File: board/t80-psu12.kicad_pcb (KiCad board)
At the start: 2 copper layers, 26 x 80 mm, 28 parts, among them J1 Conn_01x02_Female, U1 FR8205, U2 FR8205

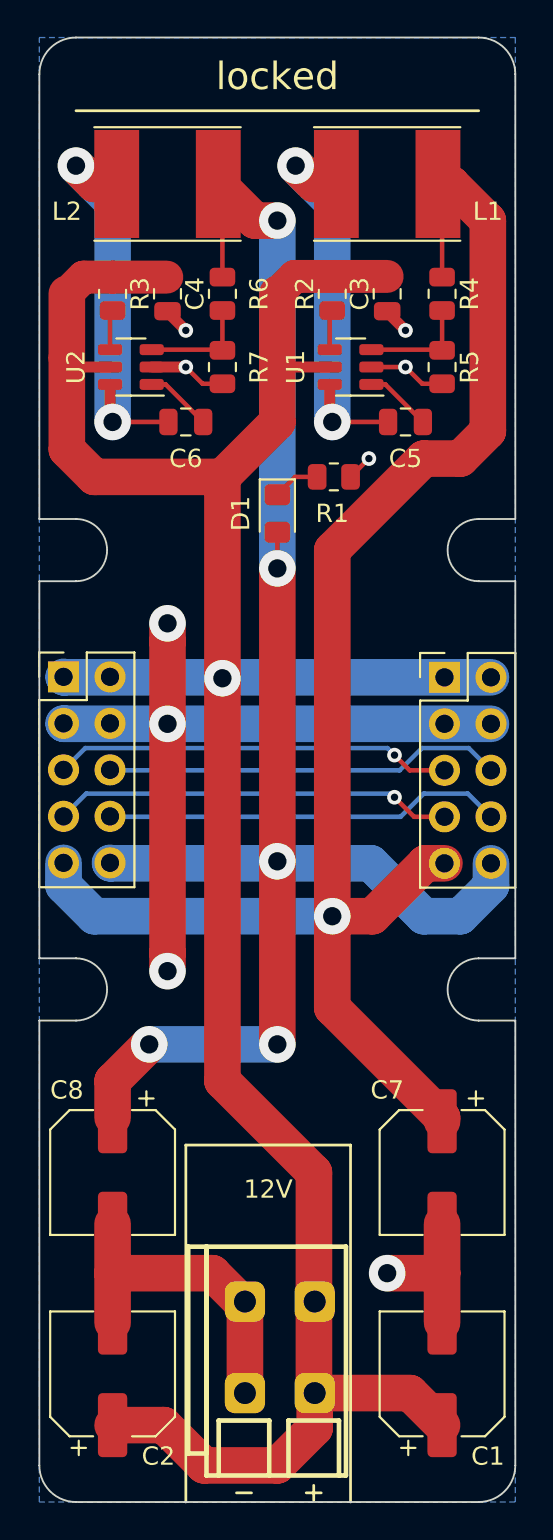
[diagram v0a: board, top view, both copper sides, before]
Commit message: WIP
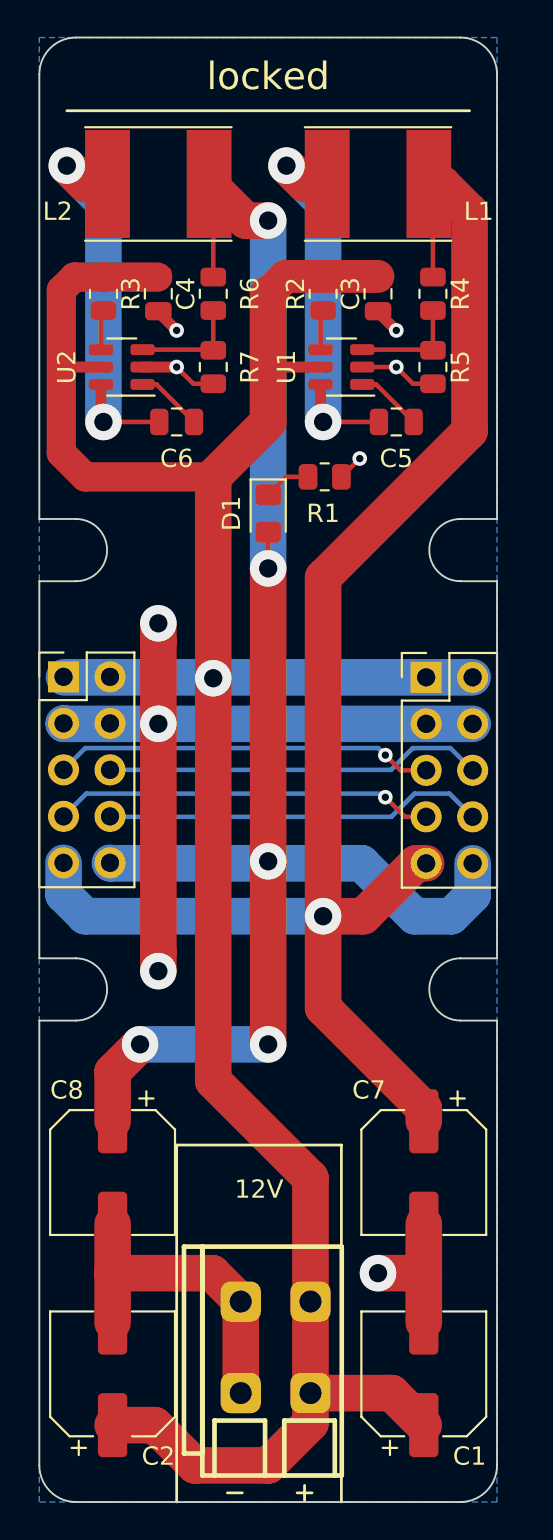
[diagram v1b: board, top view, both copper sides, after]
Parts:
- moved C1 1.00 mm to (106.0, 133.0)
- moved C7 1.00 mm to (106.0, 122.0)
- moved X2 1.00 mm to (106.1, 95.0)
- moved C3 0.50 mm to (103.5, 74.0)
- moved C4 0.50 mm to (91.5, 74.0)
- moved C5 0.50 mm to (104.5, 81.0)
- moved C6 0.50 mm to (92.5, 81.0)
- moved D1 0.50 mm to (97.5, 86.0)
- moved L1 0.50 mm to (103.5, 68.0)
- moved L2 0.50 mm to (91.5, 68.0)
- moved NT1 0.50 mm to (94.5, 95.0)
- moved NT2 0.50 mm to (100.5, 108.0)
- moved NT3 0.50 mm to (97.5, 105.0)
- moved NT4 0.50 mm to (91.5, 97.5)
- moved NT5 0.50 mm to (91.5, 97.5)
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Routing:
- net +5V: track 65.1 -> 63.3 mm
- net +12V: track 121.0 -> 119.3 mm
- net /PWR_LINE_12V: track 23.4 -> 22.3 mm
- net /SDA: track 21.8 -> 20.8 mm
- net /SCL: track 21.8 -> 20.8 mm
- net /IRQ: track 21.9 -> 20.9 mm
- net /RST: track 21.9 -> 20.9 mm
- net /PWR_LINE_GND: track 23.4 -> 22.4 mm
- net /PWR_LINE_5V: track 23.9 -> 23.2 mm
- net /PWR_LINE_3V3: track 23.9 -> 23.2 mm
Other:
- board size 26 x 80 mm -> 25 x 80 mm
